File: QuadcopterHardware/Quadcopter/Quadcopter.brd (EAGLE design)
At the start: 47 x 28 mm, 47 parts, among them J2 FTDI_DEVICERA_SMT, M1 WIRELESS-NRF24L01, U1 ATMEGA328P_TQFP, U3 GY-521MPU6050

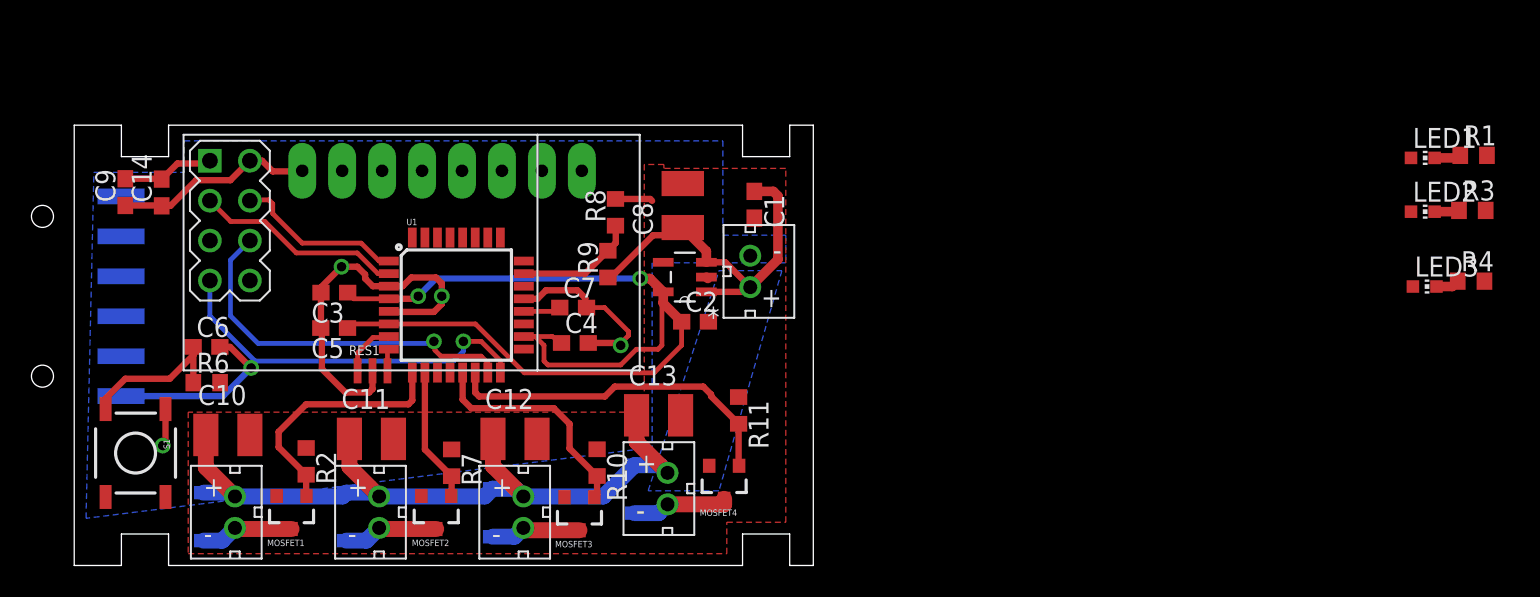
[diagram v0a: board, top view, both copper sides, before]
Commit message: getting there
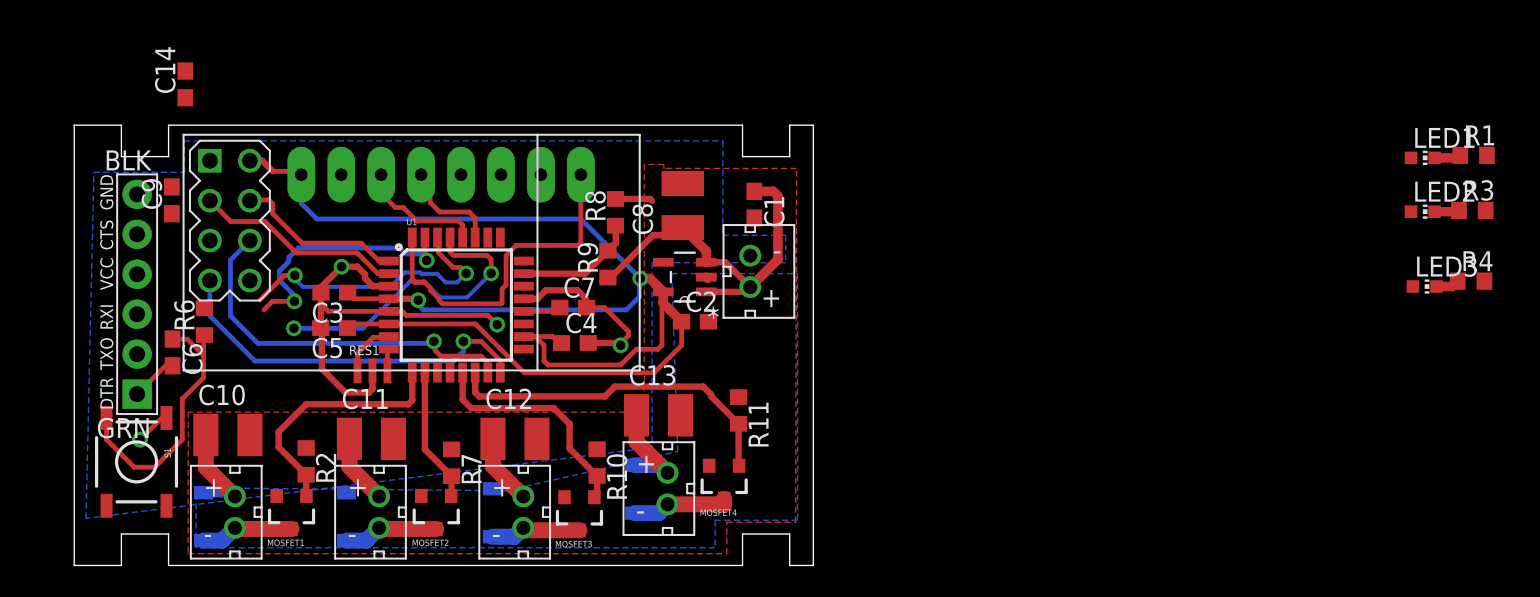
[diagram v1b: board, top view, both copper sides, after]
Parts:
- removed J2: FTDI_DEVICERA_SMT, quad:FTDI_DEVICE_RA_SMT
- added J1: FTDI_DEVICE, quad:FTDI_DEVICE_SIDE
- moved C14 7.04 mm to (7.06, 30.6)
- moved R6 3.88 mm to (8.28, 15.5), turned to 90 degrees
- moved C9 3.01 mm to (6.21, 23.2)
- moved C6 2.19 mm to (6.25, 13.5), turned to 270 degrees
- moved S1 0.57 mm to (3.96, 6.59)
- moved U3 0.26 mm to (23.3, 16.0)
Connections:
- net 3V3: now also J1.P$4; no longer J2.4
- net DTR: now also J1.P$1; no longer J2.1
- net GND: now also J1.P$5, J1.P$6; no longer J2.5, J2.6
- net UART_RX: now also J1.P$3; no longer J2.3
- net UART_TX: now also J1.P$2; no longer J2.2
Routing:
- net RST: track 9.72 -> 36.7 mm, vias 0 -> 2
- net VBATT: track 73.2 -> 47.4 mm
- net ACC_INT: track 0.00 -> 21.7 mm
- net UART_RX: track 0.00 -> 18.4 mm, vias 0 -> 2
- net 3V3: track 77.6 -> 95.3 mm
- net UART_TX: track 0.00 -> 16.6 mm, vias 0 -> 2
- net DTR: track 11.6 -> 3.00 mm, vias 1 -> 0
- net SCL: track 0.00 -> 8.02 mm
- net SDA: track 0.00 -> 6.52 mm
- net GND: track 46.9 -> 44.3 mm

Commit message: draft 1 done, needs checking
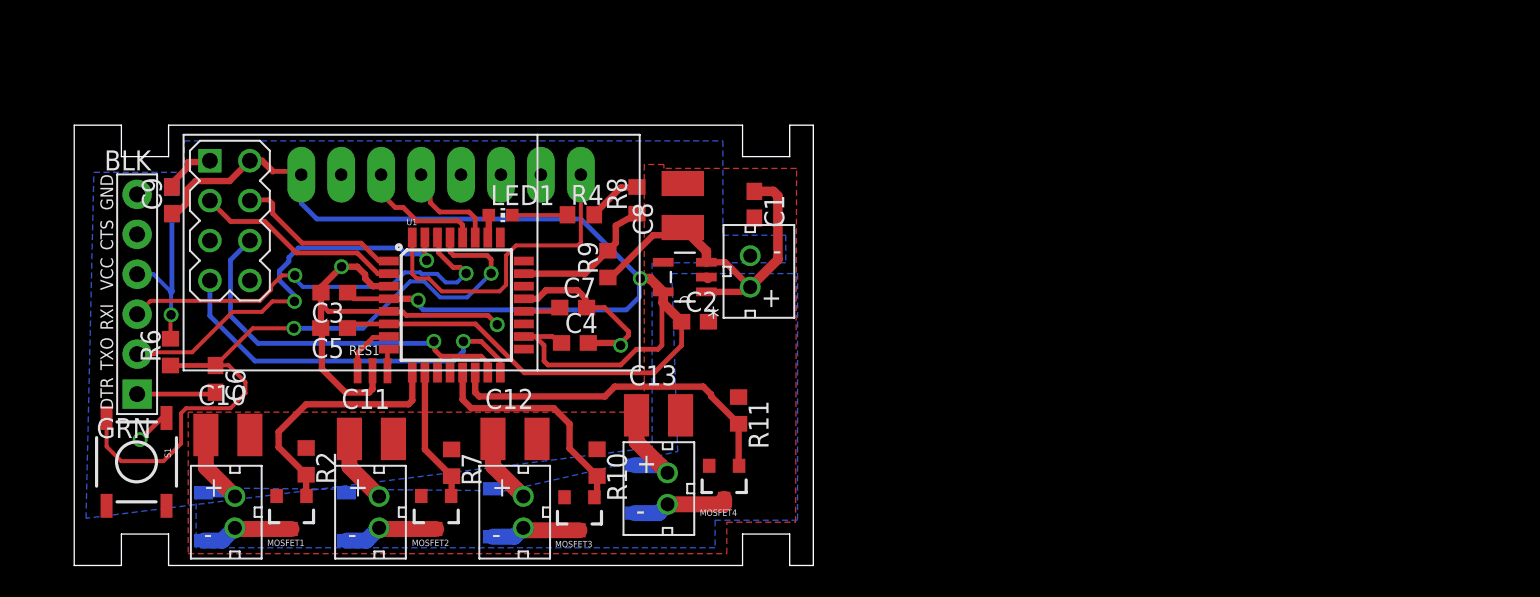
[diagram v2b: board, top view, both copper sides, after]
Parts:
- removed LED2, LED3: RED, led:CHIP-LED0603
- removed R1, R3: 150, rcl:R0603
- moved LED1 58.8 mm to (27.1, 22.3)
- moved R4 56.8 mm to (32.2, 22.3)
- moved C14 7.42 mm to (6.21, 23.2), flipped to the bottom
- moved C6 3.21 mm to (8.98, 11.9)
- moved R6 2.90 mm to (6.12, 13.6)
- moved R8 1.56 mm to (35.8, 23.2)
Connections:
- removed net LED2: LED2.A, U1.25
- removed net LED3: LED3.A, U1.26
- removed net N$2: LED2.C, R3.1
- removed net N$3: LED3.C, R4.1
- removed net N$5: LED1.C, R1.1
- new net LEDRESISTOR: LED1.C, R4.1
- net GND: no longer R1.2, R3.2
- net LED1: now also U1.26; no longer U1.24
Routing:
- net 3V3: track 95.3 -> 112.7 mm, vias 2 -> 3
- net UART_TX: track 16.6 -> 25.7 mm
- net RST: track 36.7 -> 45.3 mm
- net UART_RX: track 18.4 -> 26.7 mm
- net GND: track 44.3 -> 48.5 mm
- net LEDRESISTOR: track 0.00 -> 3.52 mm
- net DTR: track 3.00 -> 5.03 mm
- net N$5: track 1.70 -> 0.00 mm
- net N$2: track 1.58 -> 0.00 mm
- net VDIV: track 7.76 -> 9.30 mm
- net ACC_INT: track 21.7 -> 20.2 mm
- net N$3: track 1.49 -> 0.00 mm
- net LED1: track 0.00 -> 1.37 mm
